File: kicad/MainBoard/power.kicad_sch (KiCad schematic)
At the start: 75 parts, among them J20 USB_C_Receptacle, Q16 AO3401A, Q17 AO3400A, SW1 SW_SPDT, U13 BQ27441-G1, U14 HY2111-GB, U15 FS8205A, U17 TPS61088, U2 BQ25601, U26 SN74LVC1G3157DCKR, U27 SN74LVC1G3157DCKR

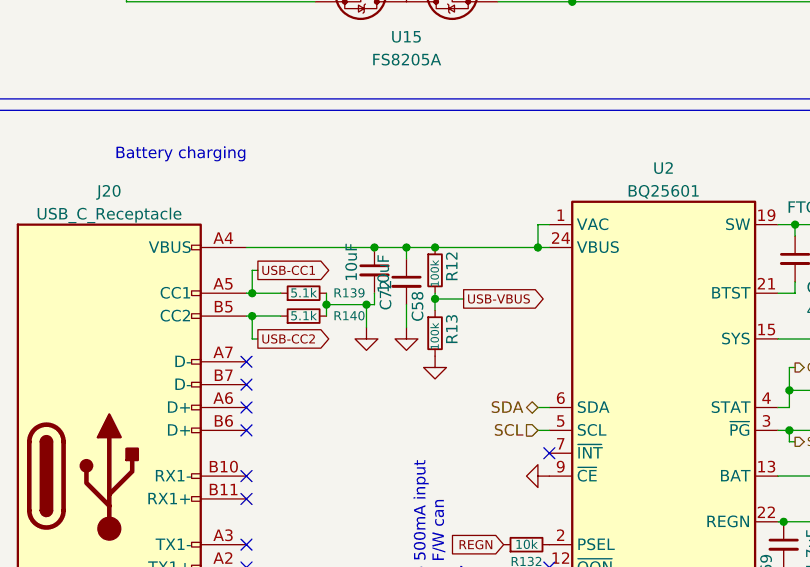
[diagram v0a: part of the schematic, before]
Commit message: tweaks
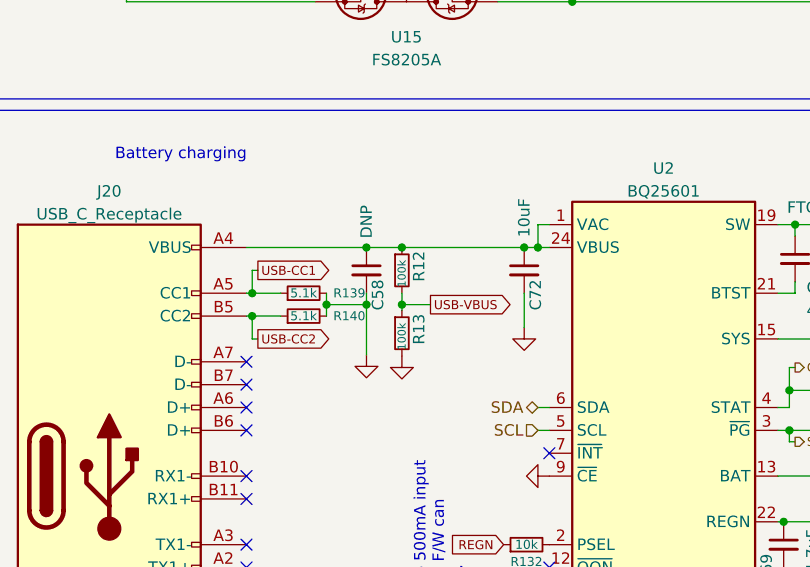
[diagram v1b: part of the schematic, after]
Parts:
- C58: value 10uF -> DNP; LCSC C19702 -> (none)
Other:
- moved on the sheet: C58, C72, R12, R13
